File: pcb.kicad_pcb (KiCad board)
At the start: 4 copper layers, 26 x 30 mm, 71 parts, among them J1 Conn_ARM_SWD_TagConnect_TC203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, J2 Conn_ARM_JTAG_SWD_10, J3 JST B04B-PASK, P1 USB_C_Plug, Q1 AO3400A, Q2 AO3400A, Q3 AO3401A, Q4 AO3401A, SW1 SW_Push, U1 WE-TVS-82400102, U2 STM32F103C8T6, U5 74LVC2T45DC, U6 74LVC2T45DC, U7 74LVC2T45DC, U8 74LVC2T45DC, U9 AP2112K-3.3, Y1 8MHz

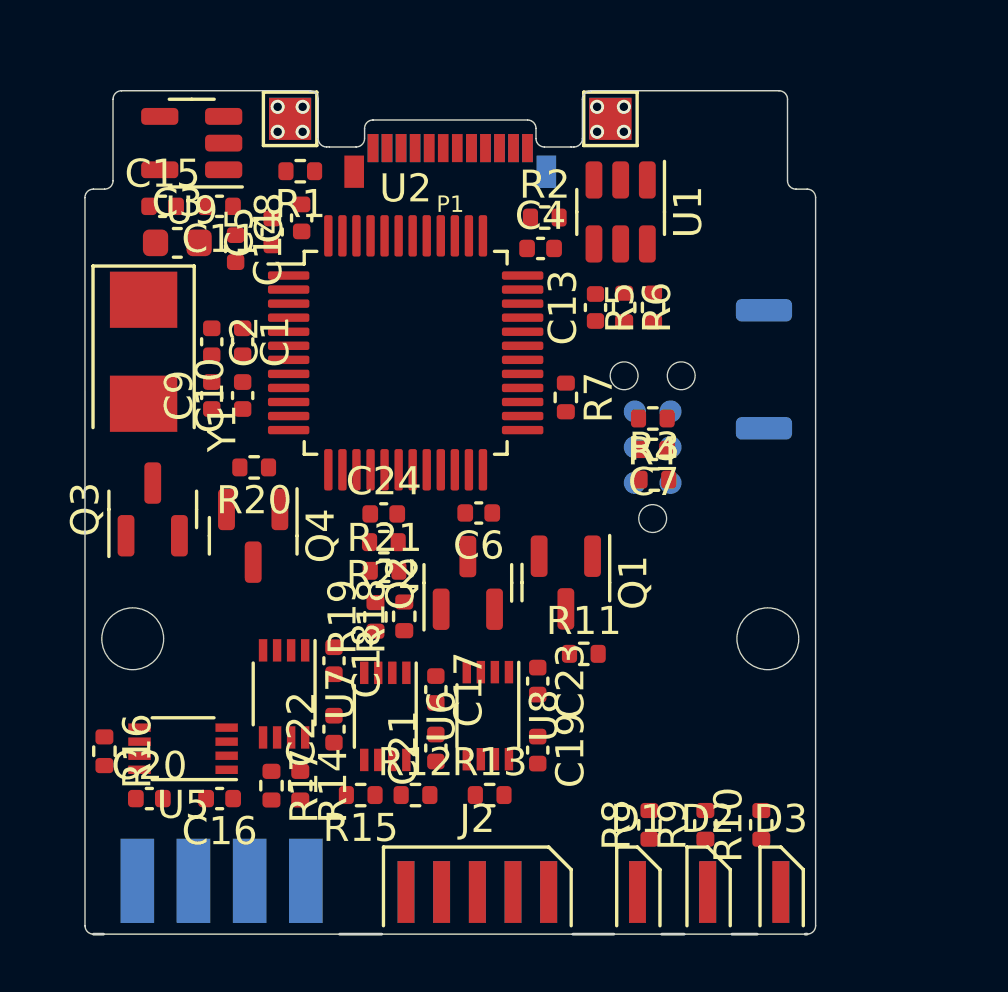
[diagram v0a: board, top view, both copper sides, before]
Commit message: Layout and routing
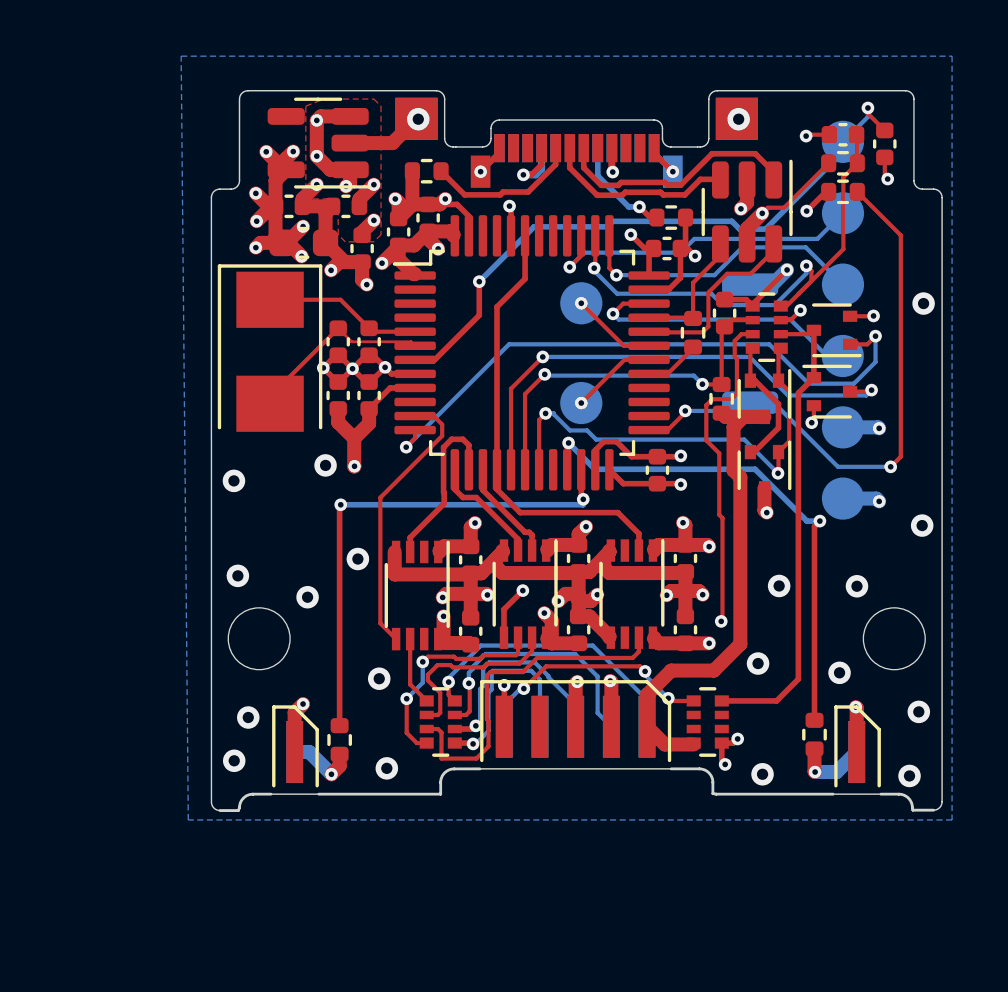
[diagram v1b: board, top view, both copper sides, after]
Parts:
- removed C16, C20: 100n, Capacitor_SMD:C_0402_1005Metric
- removed D1: Yellow, Connectors:LED_THT_Edge Mount
- removed J1: Conn_ARM_SWD_TagConnect_TC2030-NL, Connector:Tag-Connect_TC2030-IDC-NL_2x03_P1.27mm_Vertical
- removed J3: JST B04B-PASK, Connectors:JST B04B-PASK Edge Mount
- removed Q3, Q4: AO3401A, Package_TO_SOT_SMD:SOT-23
- removed R11, R12, R13, R14, R15, R16, R17, R19: 100R, Resistor_SMD:R_0402_1005Metric
- removed R18, R20, R22, R6: 10k, Resistor_SMD:R_0402_1005Metric
- removed R3: 0R, Resistor_SMD:R_0402_1005Metric
- removed R8: 330R, Resistor_SMD:R_0402_1005Metric
- removed U5: 74LVC2T45DC, Package_SO:VSSOP-8_2.3x2mm_P0.5mm
- added G***: LOGO, framework-debug-probe:pretzel, B.Cu at (132.4, 86.5)
- added NT1: NetTie_2, NetTie:NetTie-2_SMD_Pad0.5mm, F.Cu at (133.9, 84.5)
- added Q5: 2N7002, Package_TO_SOT_SMD:SOT-523, F.Cu at (150.9, 80.1)
- added Q6: 2N7002, Package_TO_SOT_SMD:SOT-523, F.Cu at (150.9, 82.3)
- added RN1: 121R, Resistor_SMD:R_Array_Convex_4x0402, F.Cu at (137.0, 94.0)
- added RN2: 121R, Resistor_SMD:R_Array_Convex_4x0402, F.Cu at (146.5, 94.0)
- added RN3: 10k, Resistor_SMD:R_Array_Convex_4x0402, F.Cu at (148.6, 80.0)
- added TP10: TestPoint, TestPoint:TestPoint_Pad_D1.5mm, B.Cu at (151.3, 86.1)
- added TP11: TestPoint, TestPoint:TestPoint_Pad_D1.5mm, B.Cu at (142.0, 82.7)
- added TP12: TestPoint, TestPoint:TestPoint_Pad_D1.5mm, B.Cu at (142.0, 79.2)
- added TP5: TestPoint, TestPoint:TestPoint_Pad_D1.5mm, B.Cu at (151.3, 73.4)
- added TP6: TestPoint, TestPoint:TestPoint_Pad_D1.5mm, B.Cu at (151.3, 78.5)
- added TP7: TestPoint, TestPoint:TestPoint_Pad_D1.5mm, B.Cu at (151.3, 81.0)
- added TP8: TestPoint, TestPoint:TestPoint_Pad_D1.5mm, B.Cu at (151.3, 75.9)
- added TP9: TestPoint, TestPoint:TestPoint_Pad_D1.5mm, B.Cu at (151.3, 83.6)
- Q1, Q2: value AO3400A -> CJE3139K; footprint Package_TO_SOT_SMD:SOT-23 -> Package_TO_SOT_SMD:SOT-523
- moved D3 18.0 mm to (131.8, 95.1)
- moved R10 15.3 mm to (133.4, 94.7), turned to -90 degrees
- moved C24 14.1 mm to (147.1, 79.5), turned to 90 degrees
- moved C7 13.6 mm to (152.8, 73.5), turned to -90 degrees
- moved R21 13.5 mm to (147.0, 82.5), turned to -90 degrees
- moved C18 13.0 mm to (145.7, 88.2)
- moved C22 13.0 mm to (145.7, 90.8)
- moved U7 12.9 mm to (143.8, 89.5)
- moved Q2 12.4 mm to (148.5, 82.5), turned to -90 degrees
- moved C13 10.7 mm to (151.3, 73.2), turned to 180 degrees
- moved R4 10.5 mm to (151.3, 75.2)
- moved R5 8.48 mm to (151.3, 74.2), turned to 180 degrees
- moved Q1 8.12 mm to (148.5, 85.1)
- moved D2 7.27 mm to (151.8, 95.1)
- moved C19 7.18 mm to (138.1, 88.3)
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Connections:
- C10 pad 1: +3V3 -> VDDA
- C7 pad 1: Net-(U2-NRST) -> nRST
- C9 pad 1: +3V3 -> VDDA
- Q1 pad 1: iRST -> PWR_BR
- Q1 pad 2: GND -> Net-(RN3D-R4.1)
- Q1 pad 3: xRST -> +3V3
- Q2 pad 1: xRST -> PWR_BR
- Q2 pad 2: GND -> Net-(RN3D-R4.1)
- Q2 pad 3: RST_SENSE -> TPWR
- U2 pad 20: LED0 -> unconnected-(U2-PB2-Pad20)
- U2 pad 7: Net-(U2-NRST) -> nRST
- U2 pad 9: +3V3 -> VDDA
- U7 pad 3: iRXD -> unconnected-(U7-2A-Pad3)
- U7 pad 6: xRXD -> unconnected-(U7-2B-Pad6)
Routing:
- net GND: track 0.00 -> 78.6 mm, vias 8 -> 52
- net +3V3: track 0.00 -> 30.9 mm, vias 0 -> 20
- net nRST: track 0.00 -> 21.8 mm, vias 0 -> 2
- net iRST: track 0.00 -> 21.8 mm, vias 0 -> 2
- net xTPWR: track 0.00 -> 19.7 mm, vias 0 -> 6
- net Net-(U2-PB12): track 0.00 -> 18.6 mm, vias 0 -> 2
- net VBUS_MEAS: track 0.00 -> 18.6 mm, vias 0 -> 2
- net LED1: track 0.00 -> 18.2 mm, vias 0 -> 2
- net LED2: track 0.00 -> 17.8 mm, vias 0 -> 2
- net RST_SENSE: track 0.00 -> 17.6 mm, vias 0 -> 2
- net TPWR: track 0.00 -> 17.0 mm
- net xRST: track 0.00 -> 16.9 mm
- net PWR_BR: track 0.00 -> 16.0 mm, vias 0 -> 2
- net iTDO: track 0.00 -> 15.7 mm
- net VBUS: track 0.00 -> 15.2 mm, vias 0 -> 8
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- added copper zone on In2.Cu, net +3V3
- added copper zone on B.Cu, net GND
- added copper zone on In1.Cu, net GND
- added copper zone on F.Cu, net VBUS
- added copper zone on In2.Cu, net VBUS
- added copper zone on In2.Cu, net xTPWR
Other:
- board size 26 x 30 mm -> 26 x 25.6 mm
- board text added: "3V3"
- board text added: "BOOT"
- board text added: "ERROR"
- board text added: "Framework Debug Probe"
- board text added: "GND"
- board text added: "IDLE"
- board text added: "JTAG SWD"
- board text added: "Jack LeFevre"
- board text added: "RST"
- board text added: "RXD"
- board text added: "SWCLK"
- board text added: "SWDIO"
- board text added: "SWO"
- board text added: "TMS SWDIO TCK SWCLK TDO SWO TDI ~{RESET}"
- board text added: "TXD"
- board text added: "rev 0.1 June 2023"

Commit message: part numbers
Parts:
- R4: value 10k -> 220k
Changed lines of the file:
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@@
     (descr "Resistor SMD 0402 (1005 Metric), square (rectangular) end terminal, IPC_7351 nominal, (Body size source: IPC-SM-782 page 72, https://www.pcb-3d.com/wordpress/wp-content/uploads/ipc-sm-782a_amendment_1_and_2.pdf), generated with kicad-footprint-generator")
     (tags "resistor")
+    (property "LCSC" "C25104")
     (property "Sheetfile" "pcb.kicad_sch")
     (property "Sheetname" "")
@@
     (descr "Resistor SMD 0402 (1005 Metric), square (rectangular) end terminal, IPC_7351 nominal, (Body size source: IPC-SM-782 page 72, https://www.pcb-3d.com/wordpress/wp-content/uploads/ipc-sm-782a_amendment_1_and_2.pdf), generated with kicad-footprint-generator")
     (tags "resistor")
+    (property "LCSC" "C163826")
     (property "Sheetfile" "pcb.kicad_sch")
     (property "Sheetname" "")
@@
     (descr "Resistor SMD 0402 (1005 Metric), square (rectangular) end terminal, IPC_7351 nominal, (Body size source: IPC-SM-782 page 72, https://www.pcb-3d.com/wordpress/wp-content/uploads/ipc-sm-782a_amendment_1_and_2.pdf), generated with kicad-footprint-generator")
     (tags "resistor")
+    (property "LCSC" "C25767")
     (property "Sheetfile" "pcb.kicad_sch")
     (property "Sheetname" "")
@@
         (effects (font (size 1 1) (thickness 0.15)))
     )
-    (fp_text value "10k" (at 0 1.17) (layer "F.Fab")
+    (fp_text value "220k" (at 0 1.17) (layer "F.Fab")
         (effects (font (size 1 1) (thickness 0.15)))
     )
@@
     (descr "Resistor SMD 0402 (1005 Metric), square (rectangular) end terminal, IPC_7351 nominal, (Body size source: IPC-SM-782 page 72, https://www.pcb-3d.com/wordpress/wp-content/uploads/ipc-sm-782a_amendment_1_and_2.pdf), generated with kicad-footprint-generator")
     (tags "resistor")
+    (property "LCSC" "C881131")
     (property "Sheetfile" "pcb.kicad_sch")
     (property "Sheetname" "")
@@
     (descr "VSSOP-8 2.3x2mm Pitch 0.5mm")
     (tags "VSSOP-8 2.3x2mm Pitch 0.5mm")
+    (property "LCSC" "C2652936")
     (property "Sheetfile" "pcb.kicad_sch")
     (property "Sheetname" "")
@@
     (descr "Resistor SMD 0402 (1005 Metric), square (rectangular) end terminal, IPC_7351 nominal, (Body size source: IPC-SM-782 page 72, https://www.pcb-3d.com/wordpress/wp-content/uploads/ipc-sm-782a_amendment_1_and_2.pdf), generated with kicad-footprint-generator")
     (tags "resistor")
+    (property "LCSC" "C163826")
     (property "Sheetfile" "pcb.kicad_sch")
     (property "Sheetname" "")
@@
     (descr "Resistor SMD 0402 (1005 Metric), square (rectangular) end terminal, IPC_7351 nominal, (Body size source: IPC-SM-782 page 72, https://www.pcb-3d.com/wordpress/wp-content/uploads/ipc-sm-782a_amendment_1_and_2.pdf), generated with kicad-footprint-generator")
     (tags "resistor")
+    (property "LCSC" "C25104")
     (property "Sheetfile" "pcb.kicad_sch")
     (property "Sheetname" "")
@@
     (descr "Resistor SMD 0402 (1005 Metric), square (rectangular) end terminal, IPC_7351 nominal, (Body size source: IPC-SM-782 page 72, https://www.pcb-3d.com/wordpress/wp-content/uploads/ipc-sm-782a_amendment_1_and_2.pdf), generated with kicad-footprint-generator")
     (tags "resistor")
+    (property "LCSC" "C881131")
     (property "Sheetfile" "pcb.kicad_sch")
     (property "Sheetname" "")
@@
     (descr "VSSOP-8 2.3x2mm Pitch 0.5mm")
     (tags "VSSOP-8 2.3x2mm Pitch 0.5mm")
-    (property "Sheetfile" "pcb.kicad_sch")
-    (property "Sheetname" "")
+    (property "LCSC" "C2652936")
+    (property "Sheetfile" "pcb.kicad_sch")
+    (property "Sheetname" "")
